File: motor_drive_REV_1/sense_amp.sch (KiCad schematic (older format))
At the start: 3 parts, among them U9 AD8418ABRMZ-RL

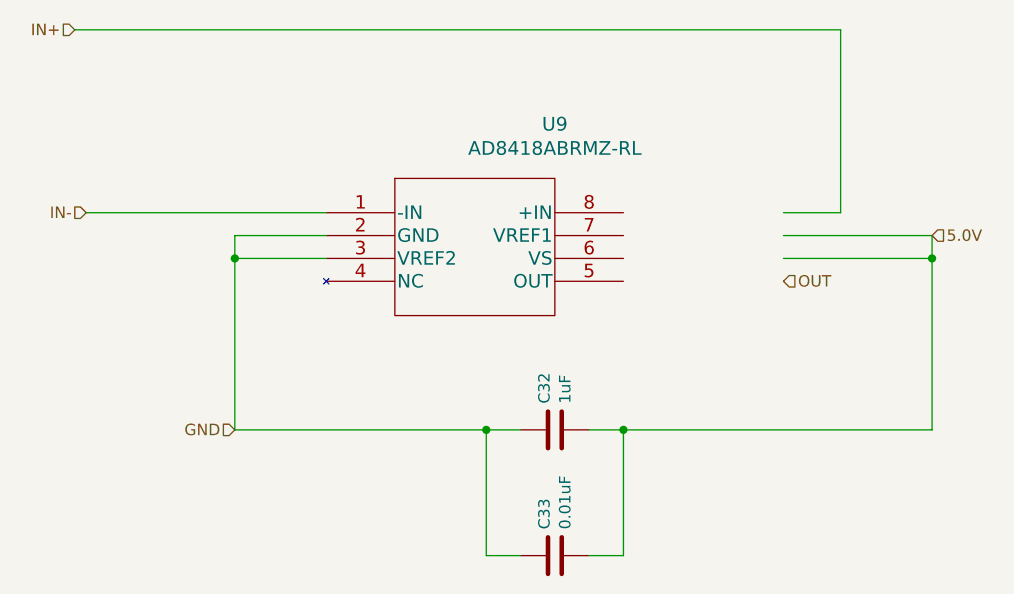
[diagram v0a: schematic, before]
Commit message: started layout
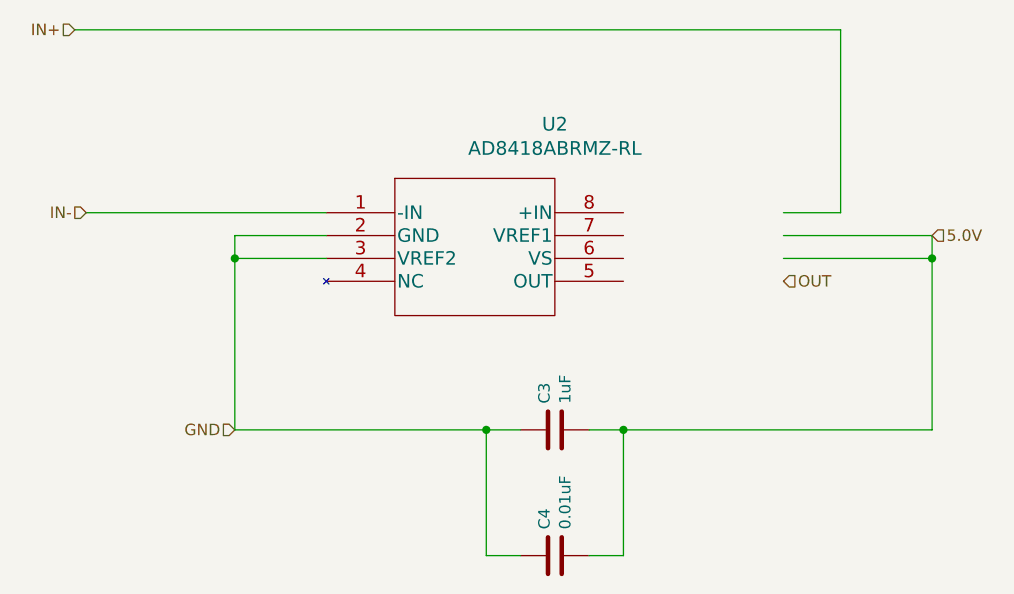
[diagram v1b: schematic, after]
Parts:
- renumbered C32 to C41, C33 to C42
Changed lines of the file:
@@
 $Descr A4 11693 8268
 encoding utf-8
-Sheet 5 14
+Sheet 6 16
 Title ""
 Date ""
@@
 AR Path="/5E33A08D/5E259F13" Ref="U4"  Part="1"
 AR Path="/5E33E36D/5E259F13" Ref="U?"  Part="1"
-F 0 "U9" H 5500 3887 60  0000 C CNN
+F 0 "U2" H 5500 3887 60  0000 C CNN
 F 1 "AD8418ABRMZ-RL" H 5500 3781 60  0000 C CNN
 F 2 "motor_drive_footprints:AD8418ABRMZ-RL" H 5500 3740 60  0001 C CNN
@@
 AR Path="/5E285F18/5E25CC80" Ref="C?"  Part="1"
 AR Path="/5E286BCF/5E25CC80" Ref="C?"  Part="1"
-AR Path="/5E291A12/5E25CC80" Ref="C32"  Part="1"
-AR Path="/5E2938C8/5E25CC80" Ref="C3"  Part="1"
-AR Path="/5E295828/5E25CC80" Ref="C5"  Part="1"
+AR Path="/5E291A12/5E25CC80" Ref="C41"  Part="1"
+AR Path="/5E2938C8/5E25CC80" Ref="C1"  Part="1"
+AR Path="/5E295828/5E25CC80" Ref="C3"  Part="1"
 AR Path="/5E2E3D6E/5E25CC80" Ref="C?"  Part="1"
 AR Path="/5E2E5BBE/5E25CC80" Ref="C?"  Part="1"
 AR Path="/5E2E7F62/5E25CC80" Ref="C?"  Part="1"
-AR Path="/5E336639/5E25CC80" Ref="C7"  Part="1"
-AR Path="/5E33A08D/5E25CC80" Ref="C9"  Part="1"
+AR Path="/5E336639/5E25CC80" Ref="C5"  Part="1"
+AR Path="/5E33A08D/5E25CC80" Ref="C7"  Part="1"
 AR Path="/5E33E36D/5E25CC80" Ref="C?"  Part="1"
-F 0 "C32" H 5615 4496 50  0000 L CNN
+F 0 "C3" H 5615 4496 50  0000 L CNN
 F 1 "1uF" H 5615 4405 50  0000 L CNN
 F 2 "motor_drive_footprints:C_0603_1608Metric" H 5538 4300 50  0001 C CNN
@@
 AR Path="/5E285F18/5E3A2D2D" Ref="C?"  Part="1"
 AR Path="/5E286BCF/5E3A2D2D" Ref="C?"  Part="1"
-AR Path="/5E291A12/5E3A2D2D" Ref="C33"  Part="1"
-AR Path="/5E2938C8/5E3A2D2D" Ref="C4"  Part="1"
-AR Path="/5E295828/5E3A2D2D" Ref="C6"  Part="1"
+AR Path="/5E291A12/5E3A2D2D" Ref="C42"  Part="1"
+AR Path="/5E2938C8/5E3A2D2D" Ref="C2"  Part="1"
+AR Path="/5E295828/5E3A2D2D" Ref="C4"  Part="1"
 AR Path="/5E2E3D6E/5E3A2D2D" Ref="C?"  Part="1"
 AR Path="/5E2E5BBE/5E3A2D2D" Ref="C?"  Part="1"
 AR Path="/5E2E7F62/5E3A2D2D" Ref="C?"  Part="1"
-AR Path="/5E336639/5E3A2D2D" Ref="C8"  Part="1"
-AR Path="/5E33A08D/5E3A2D2D" Ref="C10"  Part="1"
+AR Path="/5E336639/5E3A2D2D" Ref="C6"  Part="1"
+AR Path="/5E33A08D/5E3A2D2D" Ref="C8"  Part="1"
 AR Path="/5E33E36D/5E3A2D2D" Ref="C?"  Part="1"
-F 0 "C33" H 5615 5046 50  0000 L CNN
+F 0 "C4" H 5615 5046 50  0000 L CNN
 F 1 "0.01uF" H 5615 4955 50  0000 L CNN
 F 2 "motor_drive_footprints:C_0603_1608Metric" H 5538 4850 50  0001 C CNN

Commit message: layout
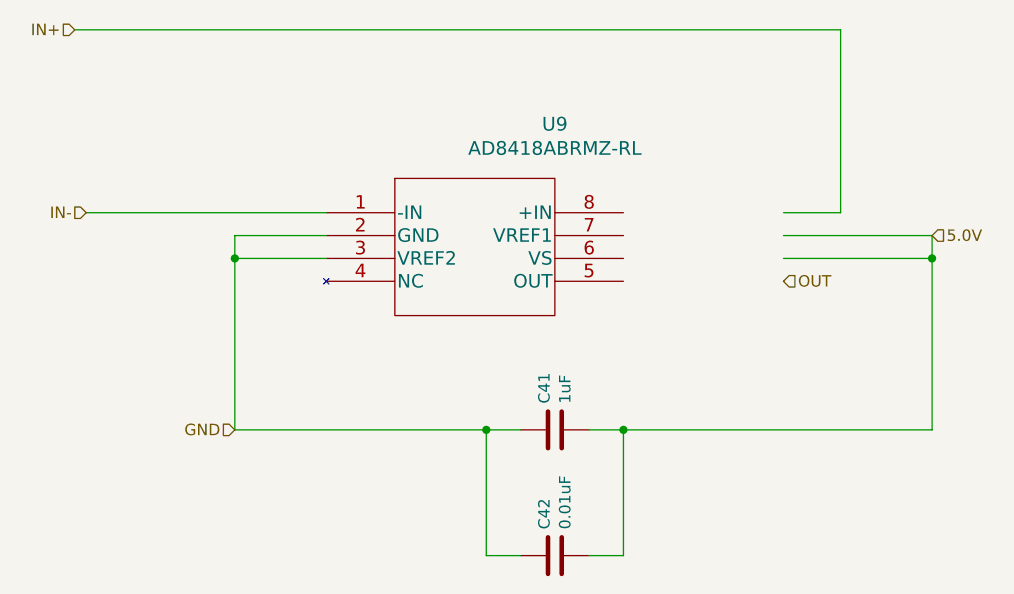
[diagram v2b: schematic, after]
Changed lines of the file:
@@
 $Descr A4 11693 8268
 encoding utf-8
-Sheet 6 16
+Sheet 14 16
 Title ""
 Date ""
@@
 AR Path="/5E33A08D/5E259F13" Ref="U4"  Part="1"
 AR Path="/5E33E36D/5E259F13" Ref="U?"  Part="1"
-F 0 "U2" H 5500 3887 60  0000 C CNN
+F 0 "U9" H 5500 3887 60  0000 C CNN
 F 1 "AD8418ABRMZ-RL" H 5500 3781 60  0000 C CNN
 F 2 "motor_drive_footprints:AD8418ABRMZ-RL" H 5500 3740 60  0001 C CNN
@@
 AR Path="/5E33A08D/5E25CC80" Ref="C7"  Part="1"
 AR Path="/5E33E36D/5E25CC80" Ref="C?"  Part="1"
-F 0 "C3" H 5615 4496 50  0000 L CNN
+F 0 "C41" H 5615 4496 50  0000 L CNN
 F 1 "1uF" H 5615 4405 50  0000 L CNN
 F 2 "motor_drive_footprints:C_0603_1608Metric" H 5538 4300 50  0001 C CNN
@@
 AR Path="/5E33A08D/5E3A2D2D" Ref="C8"  Part="1"
 AR Path="/5E33E36D/5E3A2D2D" Ref="C?"  Part="1"
-F 0 "C4" H 5615 5046 50  0000 L CNN
+F 0 "C42" H 5615 5046 50  0000 L CNN
 F 1 "0.01uF" H 5615 4955 50  0000 L CNN
 F 2 "motor_drive_footprints:C_0603_1608Metric" H 5538 4850 50  0001 C CNN

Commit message: layout
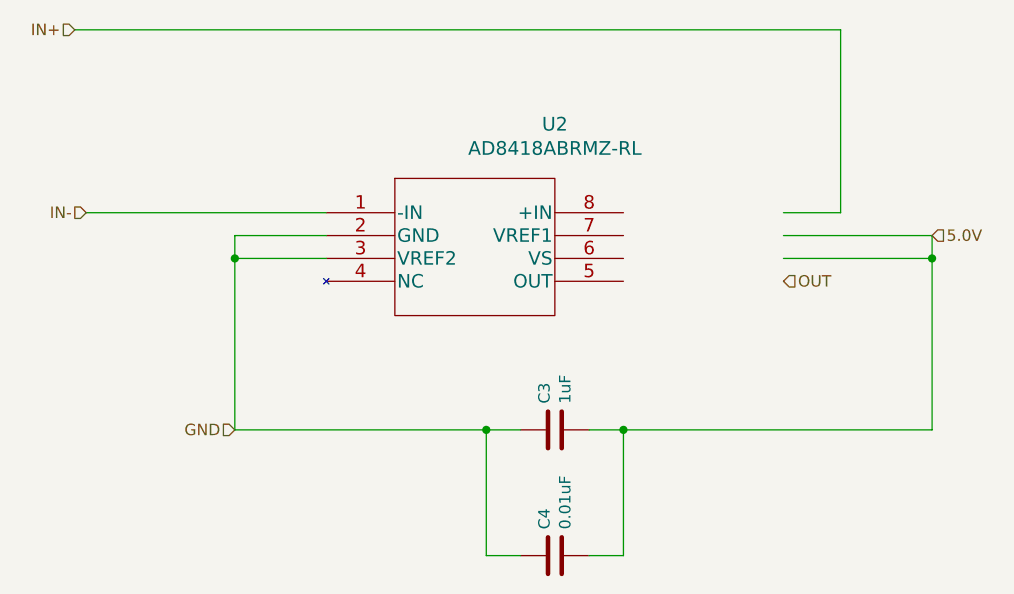
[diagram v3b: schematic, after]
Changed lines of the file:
@@
 $Descr A4 11693 8268
 encoding utf-8
-Sheet 14 16
+Sheet 6 16
 Title ""
 Date ""
@@
 AR Path="/5E33A08D/5E259F13" Ref="U4"  Part="1"
 AR Path="/5E33E36D/5E259F13" Ref="U?"  Part="1"
-F 0 "U9" H 5500 3887 60  0000 C CNN
+F 0 "U2" H 5500 3887 60  0000 C CNN
 F 1 "AD8418ABRMZ-RL" H 5500 3781 60  0000 C CNN
 F 2 "motor_drive_footprints:AD8418ABRMZ-RL" H 5500 3740 60  0001 C CNN
@@
 AR Path="/5E33A08D/5E25CC80" Ref="C7"  Part="1"
 AR Path="/5E33E36D/5E25CC80" Ref="C?"  Part="1"
-F 0 "C41" H 5615 4496 50  0000 L CNN
+F 0 "C3" H 5615 4496 50  0000 L CNN
 F 1 "1uF" H 5615 4405 50  0000 L CNN
 F 2 "motor_drive_footprints:C_0603_1608Metric" H 5538 4300 50  0001 C CNN
@@
 AR Path="/5E33A08D/5E3A2D2D" Ref="C8"  Part="1"
 AR Path="/5E33E36D/5E3A2D2D" Ref="C?"  Part="1"
-F 0 "C42" H 5615 5046 50  0000 L CNN
+F 0 "C4" H 5615 5046 50  0000 L CNN
 F 1 "0.01uF" H 5615 4955 50  0000 L CNN
 F 2 "motor_drive_footprints:C_0603_1608Metric" H 5538 4850 50  0001 C CNN
